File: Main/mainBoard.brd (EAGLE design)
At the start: 160 x 100 mm, 28 parts, among them U3 MCP2562-E/SN

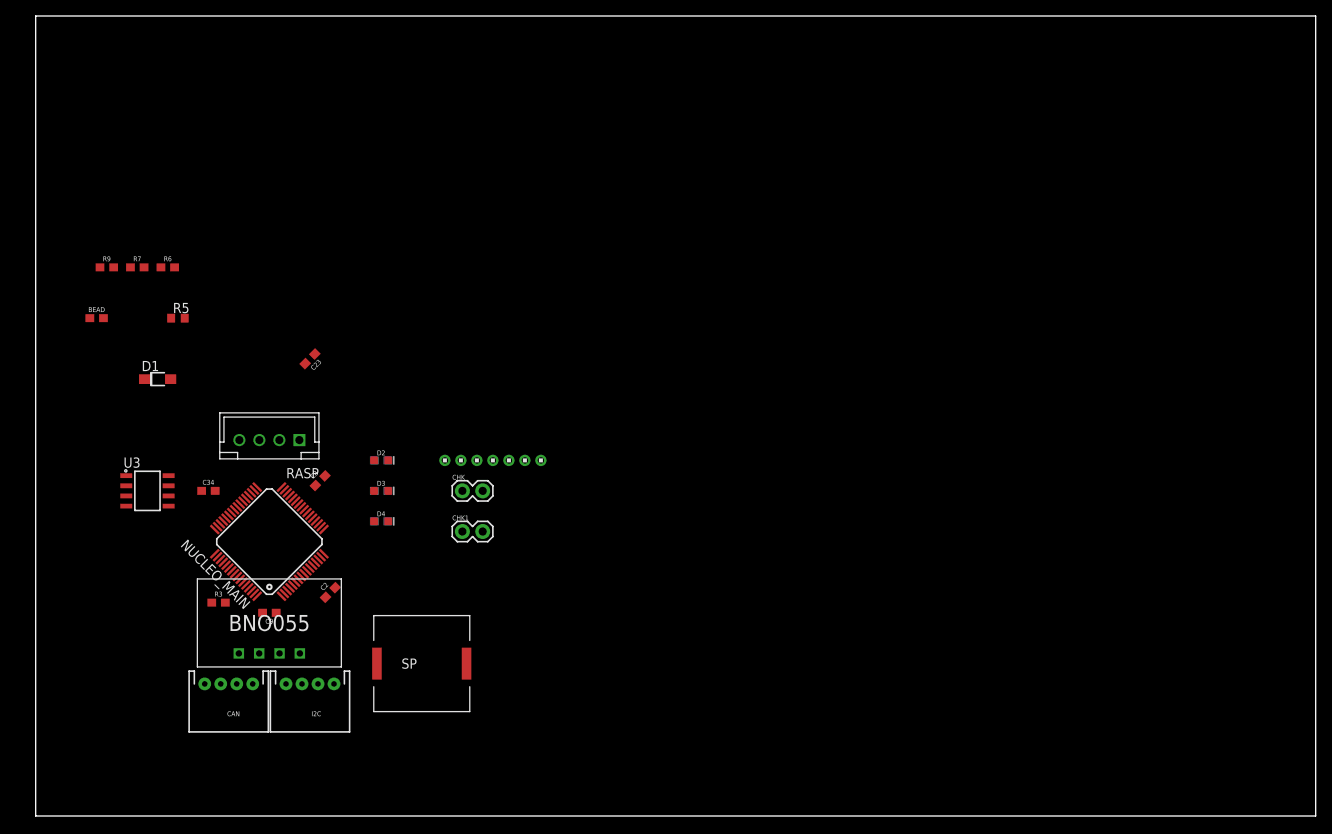
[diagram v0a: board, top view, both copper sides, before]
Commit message: some update 部品配置
# ==== Emojis ====
# ✨ :sparkles: Add new feature
# ✅  :white_check_mark: Update existing feature (not bug)
# ⚠️  :warning: Fix bug/error
# 🔥  :fire: Remove files or features
# ✏️ :pencil2: Fix typos
# 📝  :memo: Update documentation
# ♻️  :recycle: Dependencies update
# 🐧  :penguin: Improved the Linux
# 🍎  :apple: Improved the macOS
# 🔖 :bookmark: Add new library
# 🎉  :tada: Initial commit

# ==== Format ====
# :emoji: Subject
#
# Commit body...

# ==== Messages ====
# 新規(ファイル)機能追加: Add
# 機能修正、既存機能追加（バグではない): Update
# リファクタリング: Clean
# ファイル名変更:
# 削除など: Remove
# バグ修正: Fix
# バージョンアップ: Upgrade
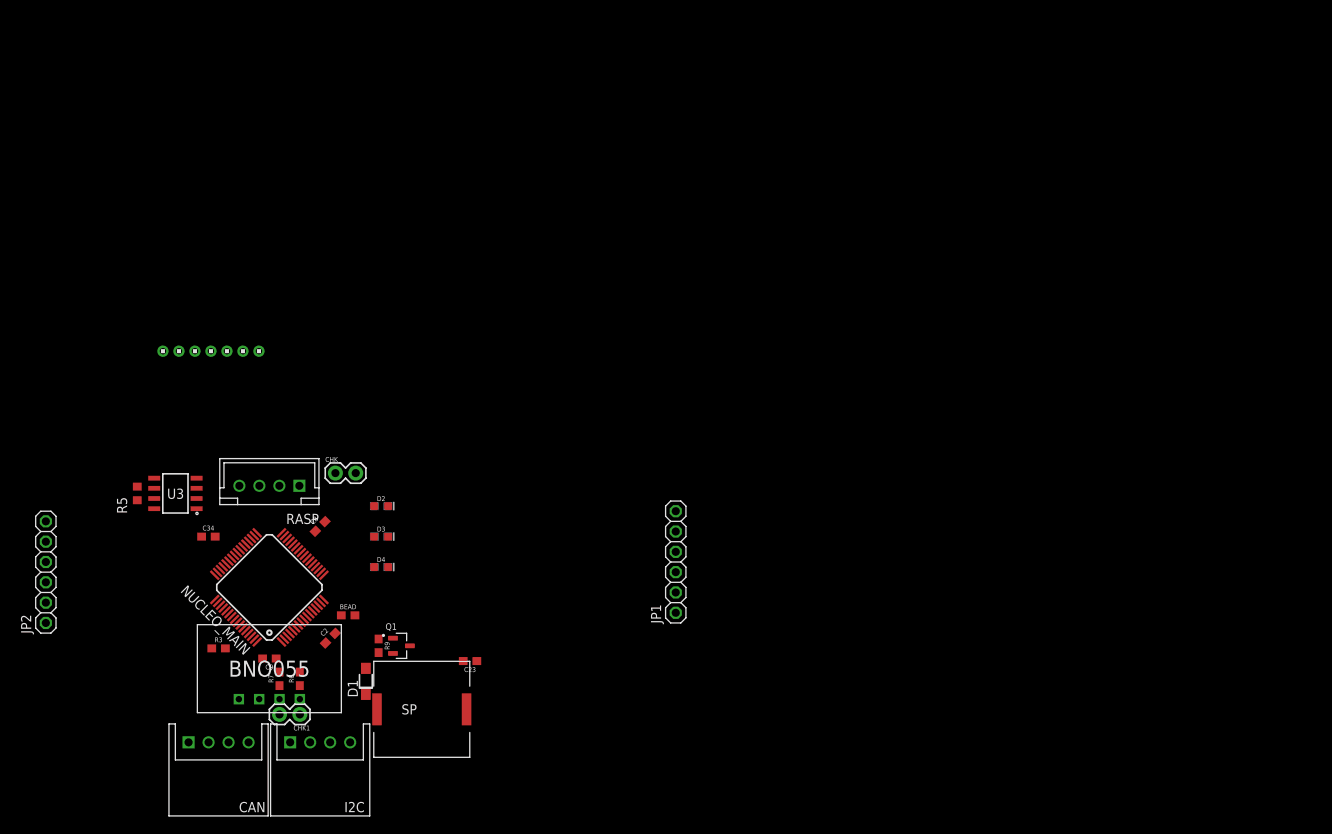
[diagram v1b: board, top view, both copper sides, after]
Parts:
- added JP1, JP2: (no value), adafruit:1X06
- added Q1: BSS138, BSS138:SOT95P240X111-3N
- CAN, I2C: device SparkFun-Connectors:JST-4-PTH -> jst-xh:S4B-XH-A
- moved R9 58.2 mm to (42.9, 21.3), turned to 270 degrees
- moved R7 54.4 mm to (30.5, 17.1), turned to 90 degrees
- moved R6 54.0 mm to (33.0, 17.1), turned to 90 degrees
- moved BEAD 48.7 mm to (39.1, 25.1)
- moved D1 45.9 mm to (41.3, 16.8), turned to 90 degrees
- moved C23 42.8 mm to (54.3, 19.4), turned to 180 degrees
- moved U$2 37.8 mm to (21.9, 58.1)
- moved CHK1 30.6 mm to (33.0, 12.7), turned to 180 degrees
- moved R5 22.5 mm to (12.7, 40.3), turned to 90 degrees
- moved CHK 16.0 mm to (37.5, 42.9)
- moved CAN 7.41 mm to (22.9, 9.21)
- moved I2C 7.41 mm to (35.6, 9.21)
- moved C34 5.72 mm to (21.6, 34.9)
- moved D2 5.72 mm to (43.2, 38.7)
- moved D3 5.72 mm to (43.2, 34.9)
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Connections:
- removed net SP: D1.C, R9.2, SP.1
- new net +15V: JP2.1
- new net GPIO0: JP1.6, NUCLEO_MAIN.PA6
- new net N$3: D1.C, SP.1
- new net N$4: D1.A, Q1.3, SP.2
- net +5V: now also JP2.2
- net BAT: now also JP1.1
- net BUZZER: now also Q1.1
- net CANH: now also CAN.1, JP1.2; no longer CAN.4
- net CANL: now also CAN.2, JP1.3; no longer CAN.3
- net DRIB_PWM: now also JP1.4
- net GND: now also CAN.3, I2C.3, JP2.4, Q1.2, R9.2; no longer CAN.2, D1.A, I2C.2, SP.2
- net KICK1: now also JP2.5
- net KICK2: now also JP2.6
- net PHOTO: now also JP1.5
- net SCL: now also I2C.2; no longer I2C.3
- net SDA: now also I2C.1; no longer I2C.4
- net VDD: now also CAN.4, I2C.4, JP2.3; no longer CAN.1, I2C.1
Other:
- board outline removed
